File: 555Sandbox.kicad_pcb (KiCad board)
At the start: 2 copper layers, 66.6 x 38 mm, 34 parts, among them J1 VIN, SW1 RESET, SW2 MODE, U1 NE555P, U2 LM3914N

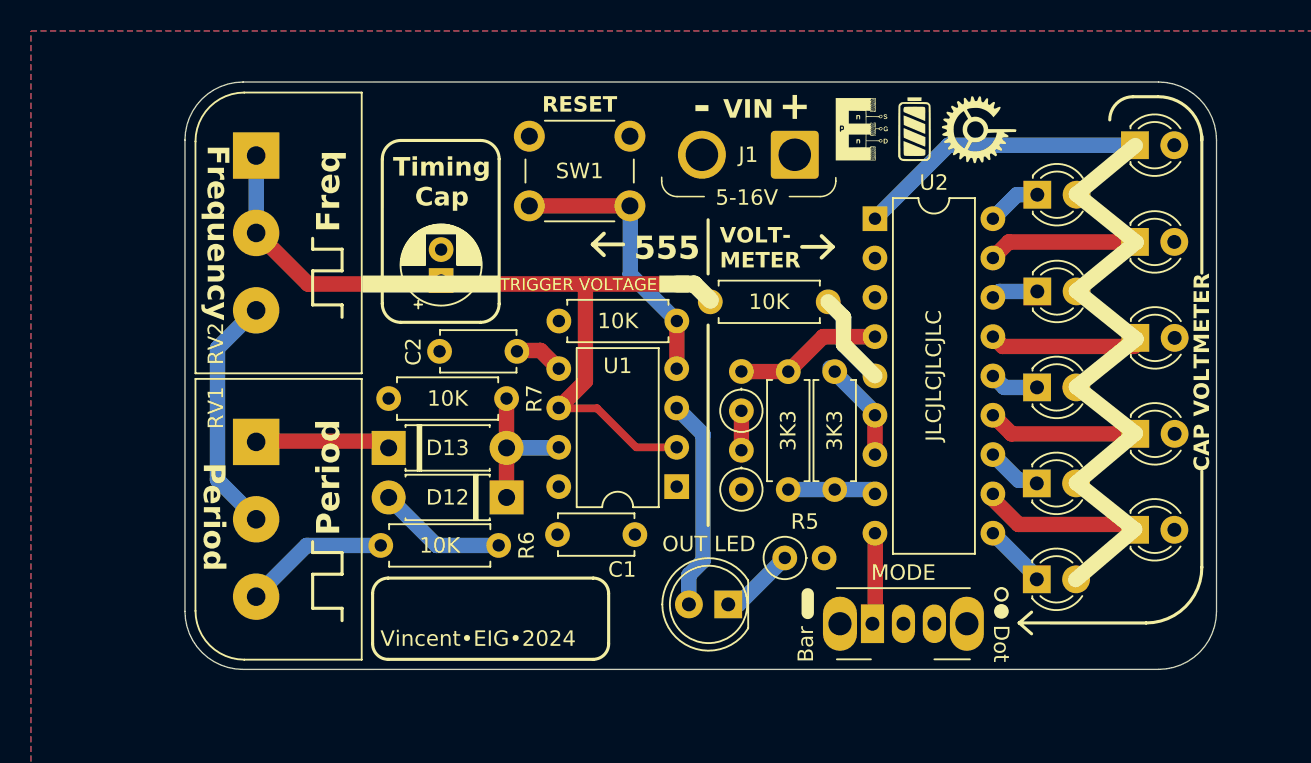
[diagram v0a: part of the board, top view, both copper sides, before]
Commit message: feat: board v1.4
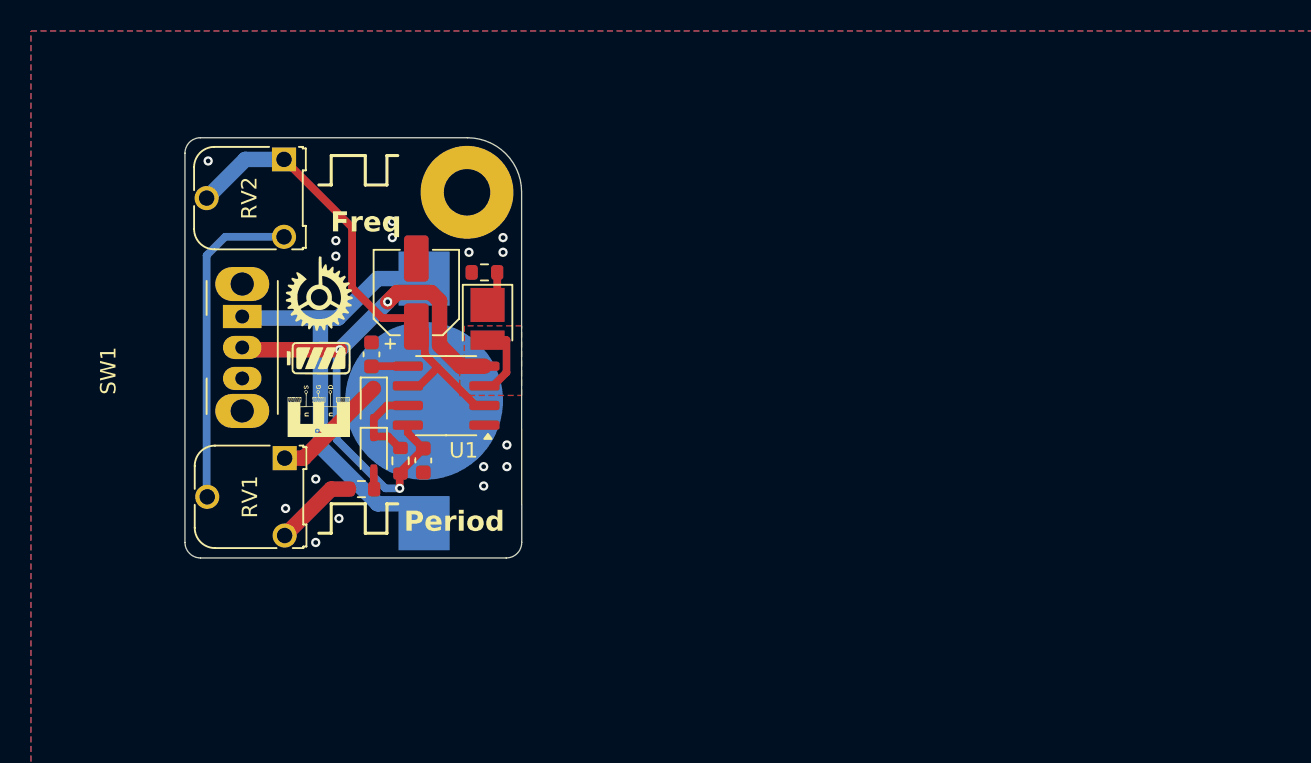
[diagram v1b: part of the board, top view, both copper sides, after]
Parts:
- removed D10, D11, D4, D5, D6, D7, D8, D9: LED, LED_THT:LED_D3.0mm
- removed D12, D13: 1N4001, Diode_THT:D_DO-41_SOD81_P7.62mm_Horizontal
- removed J1: VIN, Connector_Wire:SolderWire-1.5sqmm_1x02_P6mm_D1.7mm_OD3mm
- removed R1, R3: 10K, Resistor_THT:R_Axial_DIN0207_L6.3mm_D2.5mm_P7.62mm_Horizontal
- removed R2, R4: 3K3, Resistor_THT:R_Axial_DIN0207_L6.3mm_D2.5mm_P7.62mm_Horizontal
- removed R8, R9: 3K3, Resistor_THT:R_Axial_DIN0207_L6.3mm_D2.5mm_P2.54mm_Vertical
- removed SW2: MODE, Button_Switch_THT:SW_Slide_SPDT_Angled_CK_OS102011MA1Q
- removed U2: LM3914N, Package_DIP:DIP-18_W7.62mm
- added BT1: Battery_Cell, Battery:BatteryHolder_Keystone_3000_1x12mm, B.Cu at (90.4, 83.9)
- added G***: LOGO, NUSHSat:v1 burden bear, B.Cu at (86.5, 67.5)
- added H1: MountingHole_Pad, MountingHole:MountingHole_3mm_Pad, F.Cu at (93.2, 70.4)
- C1, C2: footprint Capacitor_THT:C_Disc_D4.7mm_W2.5mm_P5.00mm -> Capacitor_SMD:C_0603_1608Metric
- C3: value 10uF -> 4.7uF; footprint Capacitor_THT:CP_Radial_D5.0mm_P2.00mm -> Capacitor_SMD:CP_Elec_5x5.4
- D1: value OUT LED -> LED; footprint LED_THT:LED_D5.0mm -> LED_SMD:LED_PLCC_2835
- D2, D3: value LED -> 1N5819WS; footprint LED_THT:LED_D3.0mm -> Diode_SMD:D_SOD-323
- R5: value 200 -> 300; footprint Resistor_THT:R_Axial_DIN0207_L6.3mm_D2.5mm_P2.54mm_Vertical -> Resistor_SMD:R_0603_1608Metric
- R6, R7: footprint Resistor_THT:R_Axial_DIN0207_L6.3mm_D2.5mm_P7.62mm_Horizontal -> Resistor_SMD:R_0603_1608Metric
- RV1: value 100K -> 250K; footprint Potentiometer_THT:Potentiometer_Alps_RK163_Single_Horizontal -> Potentiometer_THT:Potentiometer_Runtron_RM-065_Vertical
- RV2: value 100K -> 1M; footprint Potentiometer_THT:Potentiometer_Alps_RK163_Single_Horizontal -> Potentiometer_THT:Potentiometer_Runtron_RM-065_Vertical
- SW1: value RESET -> SW_SPDT; footprint Button_Switch_THT:SW_PUSH_6mm_H4.3mm -> Button_Switch_THT:SW_Slide_SPDT_Angled_CK_OS102011MA1Q
- U1: value NE555P -> LMC555xM; footprint Package_DIP:DIP-8_W7.62mm -> Package_SO:SOIC-8_3.9x4.9mm_P1.27mm
- moved D2 51.9 mm to (87.2, 84.0), turned to -90 degrees
- moved D3 46.0 mm to (87.2, 87.2), turned to -90 degrees
- moved REF** 41.7 mm to (81.5, 86.2), turned to 90 degrees
- moved R5 26.8 mm to (94.3, 75.6), turned to 180 degrees
- moved D1 24.1 mm to (94.5, 78.6), turned to -90 degrees
- moved SW1 21.9 mm to (78.7, 78.5), turned to -90 degrees
- moved G*** 19.0 mm to (67.5, 78.7)
- moved U1 16.0 mm to (91.8, 83.6)
- moved C1 9.91 mm to (90.3, 87.8), turned to -90 degrees
- moved R6 9.59 mm to (86.3, 89.6)
- moved C2 9.40 mm to (87.0, 80.9), turned to 90 degrees
- moved R7 4.10 mm to (88.9, 87.8), turned to 90 degrees
- moved RV1 2.12 mm to (81.4, 87.6), turned to -90 degrees
- moved RV2 1.82 mm to (81.3, 68.3), turned to -90 degrees
- moved C3 1.78 mm to (89.9, 76.9)
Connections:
- D2 pad 2: VCC -> /DIS
- D3 pad 1: Net-(D3-K) -> /DIS
- D3 pad 2: VCC -> Net-(D3-A)
- R6 pad 1: Net-(D13-A) -> Net-(D3-A)
- RV1 pad 1: Net-(D12-K) -> Net-(D2-K)
- SW1 pad 1: GND -> Net-(BT1-+)
- SW1 pad 2: /RST -> VCC
- U1 pad 4: /RST -> VCC
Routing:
- net VCC: track 0.00 -> 36.9 mm, vias 0 -> 3
- net Net-(BT1-+): track 0.00 -> 28.1 mm
- net /TRIG: track 53.5 -> 31.2 mm
- net /RST: track 18.4 -> 0.00 mm
- net Net-(D2-K): track 18.8 -> 7.60 mm
- net Net-(D10-K): track 10.3 -> 0.00 mm
- net Net-(D8-K): track 9.70 -> 0.00 mm
- net Net-(D4-K): track 9.61 -> 0.00 mm
- net Net-(D6-K): track 9.42 -> 0.00 mm
- net /Voltage Meter/RLO: track 9.23 -> 0.00 mm
- net Net-(D12-K): track 8.74 -> 0.00 mm
- net /OUT: track 13.8 -> 5.10 mm
- net Net-(D13-A): track 8.39 -> 0.00 mm
- net /Voltage Meter/REF: track 6.81 -> 0.00 mm
- net Net-(U2-SIG): track 6.04 -> 0.00 mm
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- added copper zone on F.Cu, net /OUT
- added copper zone on B.Cu, net GND
- removed copper zone on B.Cu, net VCC
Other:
- board size 66.6 x 38 mm -> 21.8 x 27.1 mm
- board text added: "Designed by Vincent"
- board text added: "NUSH DSAP 2024"
- board text added: "NUSH•EIG•2024"
- board text added: "ON"
- board text added: "POWER"
- board text removed: "+"
- board text removed: "-"
- board text removed: "5-16V"
- board text removed: "555"
- board text removed: "555Sandbox"
- board text removed: "Bar"
- board text removed: "CAP VOLTMETER"
- board text removed: "Dot"
- board text removed: "Frequency"
- board text removed: "JLCJLCJLCJLC"
- board text removed: "TRIGGER VOLTAGE"
- board text removed: "Timing Cap"
- board text removed: "VOLT- METER"
- board text removed: "Vincent•EIG•2024"
